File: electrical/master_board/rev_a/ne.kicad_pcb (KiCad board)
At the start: 2 copper layers, 42.2 x 39 mm, 1 part, among them CN60 HCSR04H;F1X4

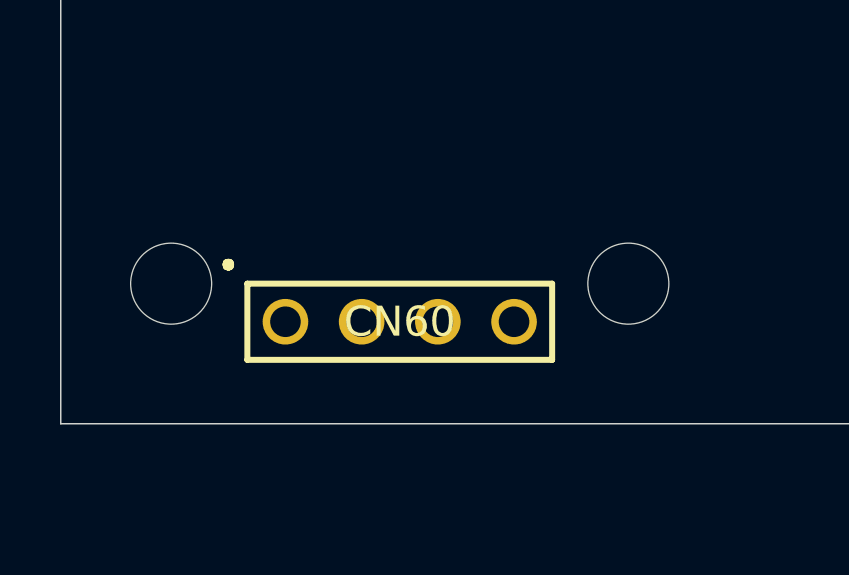
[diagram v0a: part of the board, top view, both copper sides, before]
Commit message: Another manually generate ne.kicad_pcb for debugging purposes.
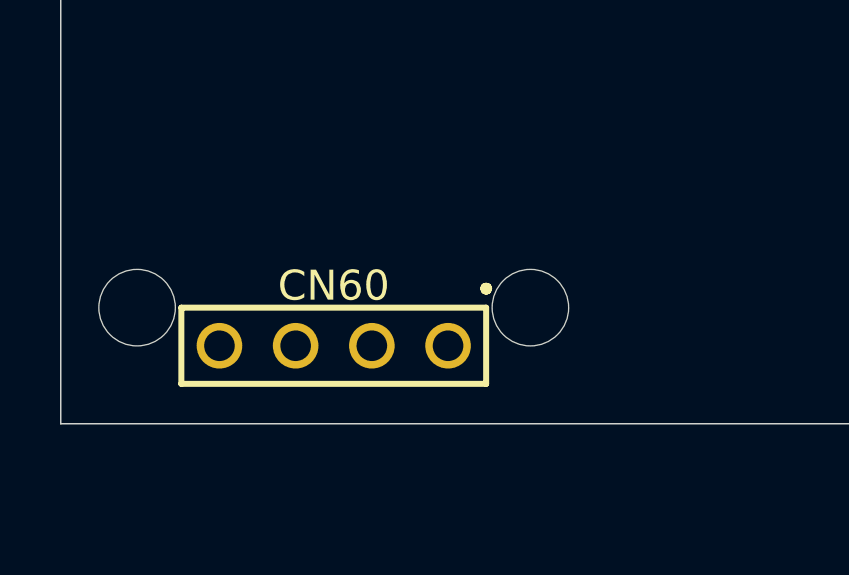
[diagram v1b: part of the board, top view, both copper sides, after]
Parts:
- CN60: value HCSR04H;F1X4 -> HCSR04;F1X4H; footprint HR2:HCSR04_F1x4H_MATE -> HR2:HCSR04_F1x4H
- moved CN60 2.34 mm to (139.1, 58.4)
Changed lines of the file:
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@@
     (add_net "Net-(CN60-Pad4)")
   )
-  (module HR2:HCSR04_F1x4H_MATE (layer F.Cu)
-    (at 141.3 57.6)
-    (fp_text reference CN60 (at 0 0) (layer F.SilkS)
+  (module HR2:HCSR04_F1x4H (layer F.Cu)
+    (at 139.1 58.4)
+    (fp_text reference CN60 (at 0 -2) (layer F.SilkS)
       (effects (font (size 1 1) (thickness 0.2)))
     )
-    (fp_text value HCSR04H;F1X4 (at 0 -2) (layer F.Fab)
+    (fp_text value HCSR04;F1X4H (at 0 0) (layer F.Fab)
       (effects (font (size 1 1) (thickness 0.2)))
     )
@@
     (fp_line (start -5.08 1.27) (end -5.08 -1.27) (layer F.SilkS) (width 0.2))
     (fp_line (start -5.08 -1.27) (end 5.08 -1.27) (layer F.SilkS) (width 0.2))
-    (fp_line (start -5.62 -1.91) (end -5.64 -1.98) (layer F.SilkS) (width 0.2))
-    (fp_line (start -5.64 -1.98) (end -5.71 -2) (layer F.SilkS) (width 0.2))
-    (fp_line (start -5.71 -2) (end -5.79 -1.98) (layer F.SilkS) (width 0.2))
-    (fp_line (start -5.79 -1.98) (end -5.81 -1.91) (layer F.SilkS) (width 0.2))
-    (fp_line (start -5.81 -1.91) (end -5.79 -1.83) (layer F.SilkS) (width 0.2))
-    (fp_line (start -5.79 -1.83) (end -5.71 -1.8) (layer F.SilkS) (width 0.2))
-    (fp_line (start -5.71 -1.8) (end -5.64 -1.83) (layer F.SilkS) (width 0.2))
-    (fp_line (start -5.64 -1.83) (end -5.62 -1.91) (layer F.SilkS) (width 0.2))
-    (pad "HCSR04 West Tie Down Hole" np_thru_hole circle (at -7.62 -1.27) (size 2.7 2.7) (drill 2.7) (layers *.Cu *.Mask))
-    (pad "HCSR04 East Tie Down Hole" np_thru_hole circle (at 7.62 -1.27) (size 2.7 2.7) (drill 2.7) (layers *.Cu *.Mask))
-    (pad 4 thru_hole circle (at 3.81 0) (size 1.52 1.52) (drill 1.02) (layers *.Cu *.Mask))
-    (pad 3 thru_hole circle (at 1.27 0) (size 1.52 1.52) (drill 1.02) (layers *.Cu *.Mask))
-    (pad 2 thru_hole circle (at -1.27 0) (size 1.52 1.52) (drill 1.02) (layers *.Cu *.Mask))
-    (pad 1 thru_hole circle (at -3.81 0) (size 1.52 1.52) (drill 1.02) (layers *.Cu *.Mask))
+    (fp_line (start 5.18 -1.91) (end 5.15 -1.98) (layer F.SilkS) (width 0.2))
+    (fp_line (start 5.15 -1.98) (end 5.08 -2) (layer F.SilkS) (width 0.2))
+    (fp_line (start 5.08 -2) (end 5.01 -1.98) (layer F.SilkS) (width 0.2))
+    (fp_line (start 5.01 -1.98) (end 4.98 -1.91) (layer F.SilkS) (width 0.2))
+    (fp_line (start 4.98 -1.91) (end 5.01 -1.83) (layer F.SilkS) (width 0.2))
+    (fp_line (start 5.01 -1.83) (end 5.08 -1.8) (layer F.SilkS) (width 0.2))
+    (fp_line (start 5.08 -1.8) (end 5.15 -1.83) (layer F.SilkS) (width 0.2))
+    (fp_line (start 5.15 -1.83) (end 5.18 -1.91) (layer F.SilkS) (width 0.2))
+    (pad "HCSR04 West Tie Down Hole" np_thru_hole circle (at -6.555 -1.27) (size 2.55 2.55) (drill 2.55) (layers *.Cu *.Mask))
+    (pad "HCSR04 East Tie Down Hole" np_thru_hole circle (at 6.555 -1.27) (size 2.55 2.55) (drill 2.55) (layers *.Cu *.Mask))
+    (pad 4 thru_hole circle (at -3.81 0) (size 1.52 1.52) (drill 1.02) (layers *.Cu *.Mask))
+    (pad 3 thru_hole circle (at -1.27 0) (size 1.52 1.52) (drill 1.02) (layers *.Cu *.Mask))
+    (pad 2 thru_hole circle (at 1.27 0) (size 1.52 1.52) (drill 1.02) (layers *.Cu *.Mask))
+    (pad 1 thru_hole circle (at 3.81 0) (size 1.52 1.52) (drill 1.02) (layers *.Cu *.Mask))
   )
   (gr_line (start 162.5 64) (end 170.67 64) (layer Edge.Cuts) (width 0.05))
